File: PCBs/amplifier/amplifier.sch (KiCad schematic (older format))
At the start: 47 parts, among them Q1 BC550, Q2 BC550, Q3 BD139, U1 LM337_TO220

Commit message: fixed schematic.
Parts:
- C1: symbol amplifier-rescue:CP -> Device:C
- C10, C2, C4, C6: symbol amplifier-rescue:CP -> Device:CP
- C3, C5, C7, C8, C9: symbol amplifier-rescue:C -> Device:C
- D1: symbol amplifier-rescue:LED -> Device:LED
- D2: symbol amplifier-rescue:D -> Device:D
- JP1: symbol amplifier-rescue:Jumper -> Device:Jumper
- Q1, Q2: symbol amplifier-rescue:BC550 -> Transistor_BJT:BC550
- Q3: symbol amplifier-rescue:BD139 -> Transistor_BJT:BD139
- R1, R10, R11, R12, R13, R14, R15, R16, R17, R18, R19, R2, R20, R21, R22, R23, R24, R25, R3, R4, R5, R6, R7, R8, R9: symbol amplifier-rescue:R -> Device:R
- RV1, RV2, RV3: symbol amplifier-rescue:POT -> Device:POT
- U1: symbol amplifier-rescue:LM337_TO220 -> Regulator_Linear:LM337_TO220
- V1: symbol amplifier-rescue:ECC88 -> Valve:ECC88
- V2: symbol amplifier-rescue:ECC83 -> Valve:ECC83
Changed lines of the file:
@@
 $EndDescr
 $Comp
-L amplifier-rescue:ECC88 V1
+L Valve:ECC88 V1
 U 1 1 5AC23A79
 P 3800 3350
@@
 $EndComp
 $Comp
-L amplifier-rescue:ECC88 V1
-U 2 1 5AC23AD8
+L Valve:ECC88 V1
+U 0 1 5AC23AD8
 P 3150 3350
 F 0 "V1" H 3320 3630 50  0000 L CNN
@@
 F 2 "Valves:VALVE-NOVAL_P" H 3420 2950 50  0001 C CNN
 F 3 "" H 3150 3350 50  0001 C CNN
-	2    3150 3350
-	1    0    0    -1
-$EndComp
-$Comp
-L amplifier-rescue:ECC88 V1
-U 3 1 5AC23B39
+	0    3150 3350
+	1    0    0    -1
+$EndComp
+$Comp
+L Valve:ECC88 V1
+U 0 1 5AC23B39
 P 10050 2950
 F 0 "V1" H 10220 3230 50  0000 L CNN
@@
 F 2 "Valves:VALVE-NOVAL_P" H 10320 2550 50  0001 C CNN
 F 3 "" H 10050 2950 50  0001 C CNN
-	3    10050 2950
-	1    0    0    -1
-$EndComp
-$Comp
-L amplifier-rescue:ECC83 V2
+	0    10050 2950
+	1    0    0    -1
+$EndComp
+$Comp
+L Valve:ECC83 V2
 U 1 1 5AC23BC0
 P 4850 2900
@@
 $EndComp
 $Comp
-L amplifier-rescue:ECC83 V2
-U 2 1 5AC23C29
+L Valve:ECC83 V2
+U 0 1 5AC23C29
 P 9250 1700
 F 0 "V2" H 9380 2010 50  0000 C CNN
@@
 F 2 "Valves:VALVE-NOVAL_P" H 9520 1300 50  0001 C CNN
 F 3 "" H 9250 1700 50  0001 C CNN
-	2    9250 1700
-	1    0    0    -1
-$EndComp
-$Comp
-L amplifier-rescue:ECC83 V2
-U 3 1 5AC23C74
+	0    9250 1700
+	1    0    0    -1
+$EndComp
+$Comp
+L Valve:ECC83 V2
+U 0 1 5AC23C74
 P 10000 1650
 F 0 "V2" H 10130 1960 50  0000 C CNN
@@
 F 2 "Valves:VALVE-NOVAL_P" H 10270 1250 50  0001 C CNN
 F 3 "" H 10000 1650 50  0001 C CNN
-	3    10000 1650
-	1    0    0    -1
-$EndComp
-$Comp
-L amplifier-rescue:R R6
+	0    10000 1650
+	1    0    0    -1
+$EndComp
+$Comp
+L Device:R R6
 U 1 1 5AC23E18
 P 3150 2700
@@
 $EndComp
 $Comp
-L amplifier-rescue:R R9
+L Device:R R9
 U 1 1 5AC24148
 P 3800 2700
@@
 $EndComp
 $Comp
-L amplifier-rescue:R R11
+L Device:R R11
 U 1 1 5AC2419C
 P 4350 2900
@@
 $EndComp
 $Comp
-L amplifier-rescue:R R3
+L Device:R R3
 U 1 1 5AC24207
 P 2400 3350
@@
 $EndComp
 $Comp
-L amplifier-rescue:R R1
+L Device:R R1
 U 1 1 5AC242C7
 P 2100 3600
@@
 $EndComp
 $Comp
-L amplifier-rescue:R R10
+L Device:R R10
 U 1 1 5AC24344
 P 4150 3550
@@
 $EndComp
 $Comp
-L amplifier-rescue:R R13
+L Device:R R13
 U 1 1 5AC243E8
 P 4750 3550
@@
 $EndComp
 $Comp
-L amplifier-rescue:R R12
+L Device:R R12
 U 1 1 5AC2443D
 P 4550 1850
@@
 $EndComp
 $Comp
-L amplifier-rescue:R R5
+L Device:R R5
 U 1 1 5AC244FB
 P 2750 4250
@@
 $EndComp
 $Comp
-L amplifier-rescue:R R2
+L Device:R R2
 U 1 1 5AC2457A
 P 2100 5650
@@
 $EndComp
 $Comp
-L amplifier-rescue:R R4
+L Device:R R4
 U 1 1 5AC245EC
 P 2500 5650
@@
 $EndComp
 $Comp
-L amplifier-rescue:R R8
+L Device:R R8
 U 1 1 5AC24637
 P 3550 5700
@@
 $EndComp
 $Comp
-L amplifier-rescue:R R7
+L Device:R R7
 U 1 1 5AC24697
 P 3550 5300
@@
 $EndComp
 $Comp
-L amplifier-rescue:R R14
+L Device:R R14
 U 1 1 5AC246EE
 P 5150 5000
@@
 $EndComp
 $Comp
-L amplifier-rescue:R R18
+L Device:R R18
 U 1 1 5AC2478C
 P 6000 5050
@@
 $EndComp
 $Comp
-L amplifier-rescue:R R16
+L Device:R R16
 U 1 1 5AC247FB
 P 5650 5400
@@
 $EndComp
 $Comp
-L amplifier-rescue:R R15
+L Device:R R15
 U 1 1 5AC2488B
 P 5450 4400
@@
 $EndComp
 $Comp
-L amplifier-rescue:R R20
+L Device:R R20
 U 1 1 5AC248FE
 P 6100 4300
@@
 $EndComp
 $Comp
-L amplifier-rescue:R R25
+L Device:R R25
 U 1 1 5AC24996
 P 7200 3700
@@
 $EndComp
 $Comp
-L amplifier-rescue:R R24
+L Device:R R24
 U 1 1 5AC24A09
 P 7200 3200
@@
 $EndComp
 $Comp
-L amplifier-rescue:R R19
+L Device:R R19
 U 1 1 5AC24A77
 P 6050 2450
@@
 $EndComp
 $Comp
-L amplifier-rescue:R R22
+L Device:R R22
 U 1 1 5AC24B04
 P 6650 2200
@@
 $EndComp
 $Comp
-L amplifier-rescue:R R21
+L Device:R R21
 U 1 1 5AC24BA2
 P 6450 2900
@@
 $EndComp
 $Comp
-L amplifier-rescue:R R23
+L Device:R R23
 U 1 1 5AC24C23
 P 7000 1600
@@
 $EndComp
 $Comp
-L amplifier-rescue:R R17
+L Device:R R17
 U 1 1 5AC24CA1
 P 5700 1150
@@
 $EndComp
 $Comp
-L amplifier-rescue:C C5
+L Device:C C5
 U 1 1 5AC24D7E
 P 4550 2000
@@
 $EndComp
 $Comp
-L amplifier-rescue:CP C1
+L Device:C C1
 U 1 1 5AC24E35
 P 1700 2400
@@
 $EndComp
 $Comp
-L amplifier-rescue:C C7
+L Device:C C7
 U 1 1 5AC25250
 P 5350 2650
@@
 $EndComp
 $Comp
-L amplifier-rescue:C C3
+L Device:C C3
 U 1 1 5AC25A48
 P 3000 5600
@@
 $EndComp
 $Comp
-L amplifier-rescue:CP C2
+L Device:CP C2
 U 1 1 5AC25B19
 P 2750 5600
@@
 $EndComp
 $Comp
-L amplifier-rescue:LM337_TO220 U1
+L Regulator_Linear:LM337_TO220 U1
 U 1 1 5AC25F95
 P 4100 5100
@@
 $EndComp
 $Comp
-L amplifier-rescue:D D2
+L Device:D D2
 U 1 1 5AC262F5
 P 4050 4800
@@
 $EndComp
 $Comp
-L amplifier-rescue:CP C4
+L Device:CP C4
 U 1 1 5AC263D7
 P 4100 5700
@@
 $EndComp
 $Comp
-L amplifier-rescue:CP C6
+L Device:CP C6
 U 1 1 5AC266B3
 P 4650 5450
@@
 $EndComp
 $Comp
-L amplifier-rescue:BC550 Q1
+L Transistor_BJT:BC550 Q1
 U 1 1 5AC26A73
 P 3050 4050
@@
 $EndComp
 $Comp
-L amplifier-rescue:BC550 Q2
+L Transistor_BJT:BC550 Q2
 U 1 1 5AC26D0A
 P 3050 4500
@@
 $EndComp
 $Comp
-L amplifier-rescue:LED D1
+L Device:LED D1
 U 1 1 5AC27322
 P 2750 4800
@@
 $EndComp
 $Comp
-L amplifier-rescue:POT RV1
+L Device:POT RV1
 U 1 1 5AC275B6
 P 3150 4900
@@
 $EndComp
 $Comp
-L amplifier-rescue:GND #PWR01
+L power:GND #PWR01
 U 1 1 5AC2ED6E
 P 5350 2850
@@
 $EndComp
 $Comp
-L amplifier-rescue:Jumper JP1
+L Device:Jumper JP1
 U 1 1 5AC2FF11
 P 5100 1850
@@
 $EndComp
 $Comp
-L amplifier-rescue:C C8
+L Device:C C8
 U 1 1 5AC305F0
 P 5650 3100
@@
 $EndComp
 $Comp
-L amplifier-rescue:C C9
+L Device:C C9
 U 1 1 5AC306D0
 P 5650 3600
@@
 $EndComp
 $Comp
-L amplifier-rescue:POT RV2
+L Device:POT RV2
 U 1 1 5AC30773
 P 5850 3350
@@
 $EndComp
 $Comp
-L amplifier-rescue:BD139 Q3
+L Transistor_BJT:BD139 Q3
 U 1 1 5AC30809
 P 6250 3350
@@
 Connection ~ 5450 3350
 $Comp
-L amplifier-rescue:POT RV3
+L Device:POT RV3
 U 1 1 5AC321F1
 P 6250 2200
@@
 Connection ~ 6450 2200
 $Comp
-L amplifier-rescue:CP C10
+L Device:CP C10
 U 1 1 5AC32FC7
 P 6450 2400
@@
 $EndComp
 $Comp
-L amplifier-rescue:GND #PWR02
+L power:GND #PWR02
 U 1 1 5AC3357B
 P 6450 2600

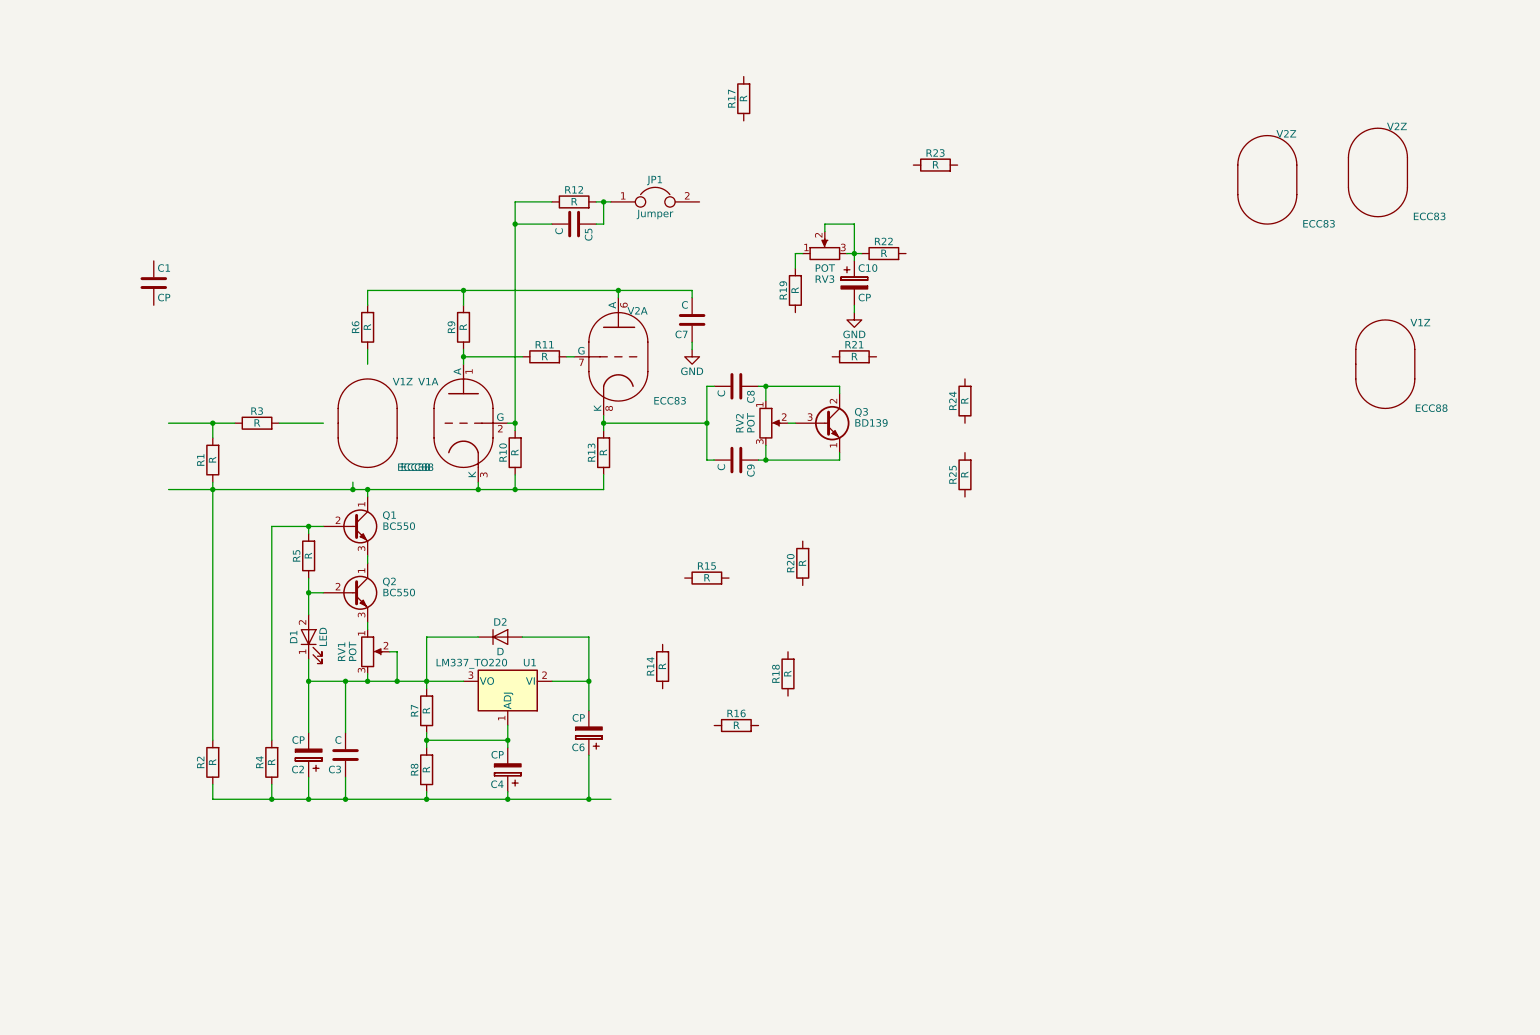
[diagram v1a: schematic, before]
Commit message: Raw finish of amp. schematic.
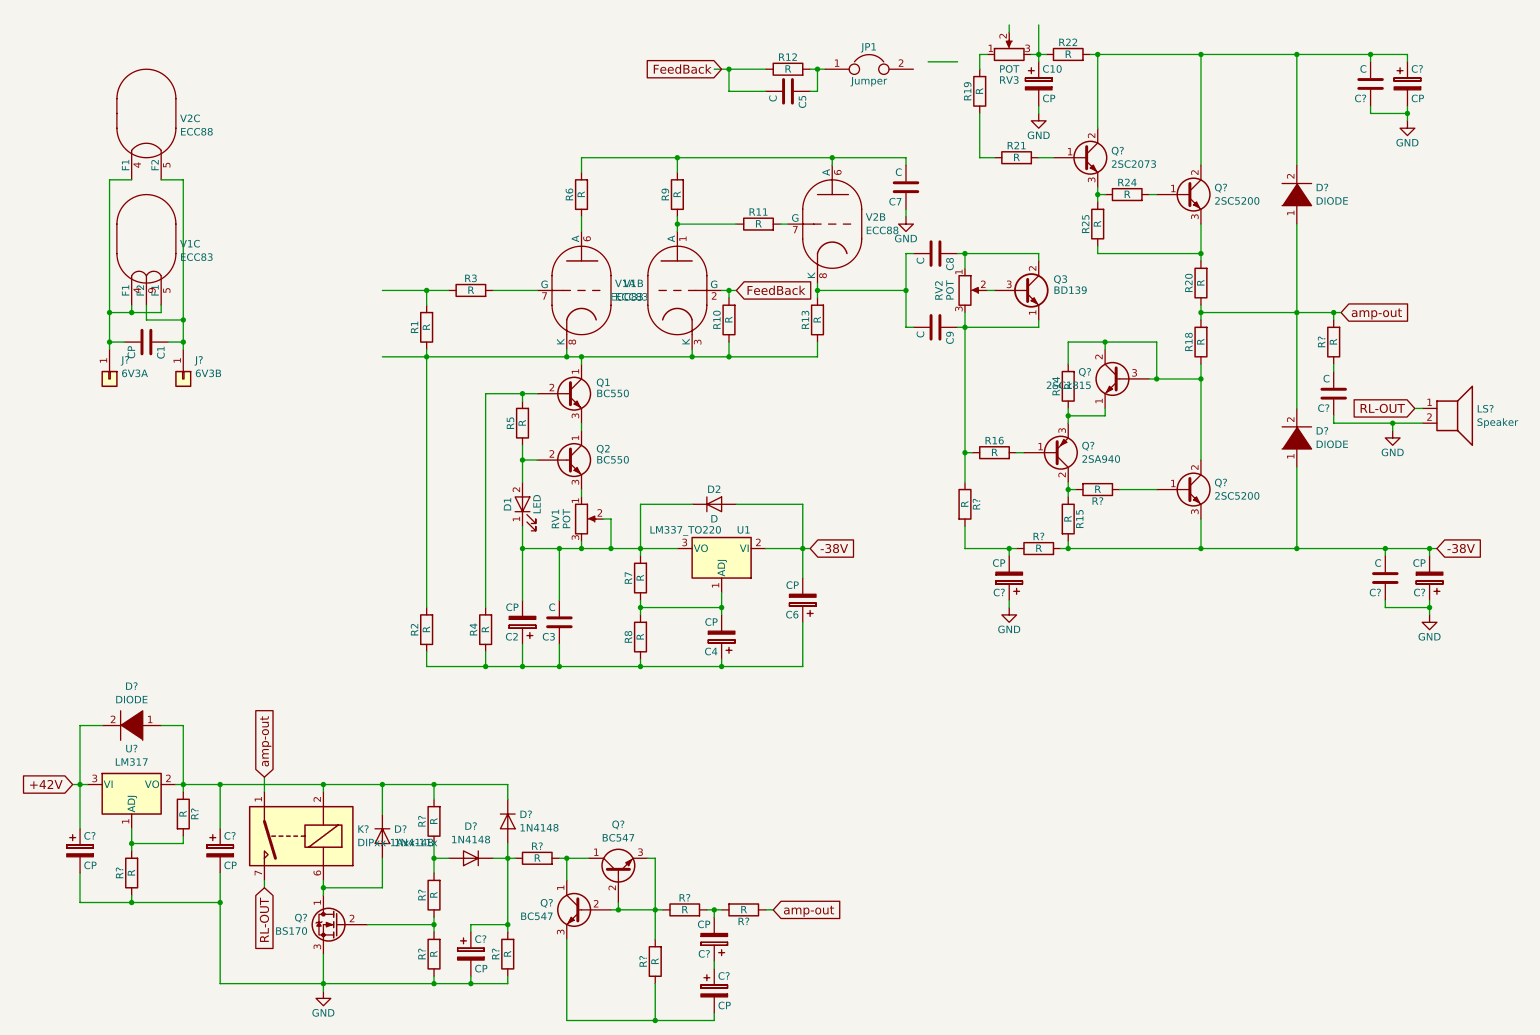
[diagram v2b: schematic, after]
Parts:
- removed R17, R23: R, symbol Device:R
- removed V1: ECC88, Valves:VALVE-NOVAL_P, symbol Valve:ECC88
- removed V2: ECC83, Valves:VALVE-NOVAL_P, symbol Valve:ECC83
- added C? (x8): CP, symbol Device:CP
- added C? (x3): C, symbol Device:C
- added D? (x3): DIODE, symbol pspice:DIODE
- added D? (x3): 1N4148, Diode_THT:D_DO-35_SOD27_P7.62mm_Horizontal, symbol Diode:1N4148
- added J?: 6V3A, symbol Connector_Generic:Conn_01x01
- added J?: 6V3B, symbol Connector_Generic:Conn_01x01
- added K?: DIPxx-1Axx-11x, Relay_THT:Relay_StandexMeder_DIP_LowProfile, symbol Relay:DIPxx-1Axx-11x
- added LS?: Speaker, symbol Device:Speaker
- added Q?: 2SC2073, symbol Device:Q_NPN_BCE
- added Q? (x2): 2SC5200, symbol Device:Q_NPN_BCE
- added Q?: 2SA940, symbol Device:Q_PNP_BCE
- added Q?: 2SC1815, Package_TO_SOT_THT:TO-92_Inline, symbol Transistor_BJT:2SC1815
- added Q?: BS170, Package_TO_SOT_THT:TO-92_Inline, symbol Transistor_FET:BS170
- added Q? (x2): BC547, Package_TO_SOT_THT:TO-92_Inline, symbol Transistor_BJT:BC547
- added R? (x14): R, symbol Device:R
- added U?: LM317, symbol Regulator_Linear:LM317_3PinPackage
- added V1: ECC83, Valve:Valve_Noval_P, symbol Valve:ECC83
- added V2: ECC88, Valve:Valve_Noval_P, symbol Valve:ECC88
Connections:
- net labels added: +42V, -38V, FeedBack, RL-OUT, amp-out
- wire segments 111 -> 285
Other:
- moved on the sheet: C1, C10, C2, C3, C4, C5, C6, C7, C8, C9, D1, D2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
